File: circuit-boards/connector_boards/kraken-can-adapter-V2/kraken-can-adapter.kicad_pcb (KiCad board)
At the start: 2 copper layers, 44.3 x 25.3 mm, 4 parts, among them J1 CAN, J2 CAN, J3 CAN_L, J4 CAN_H

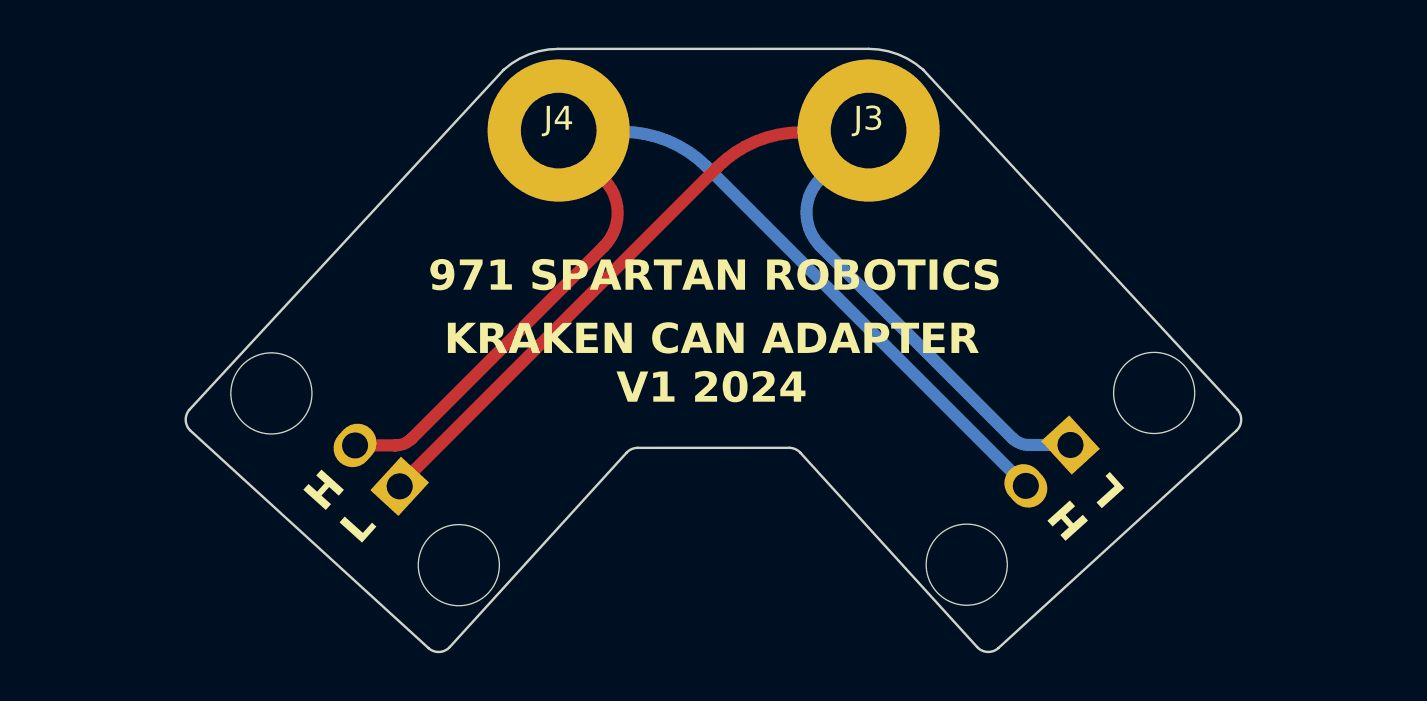
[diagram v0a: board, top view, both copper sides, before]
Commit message: Kraken Can V2
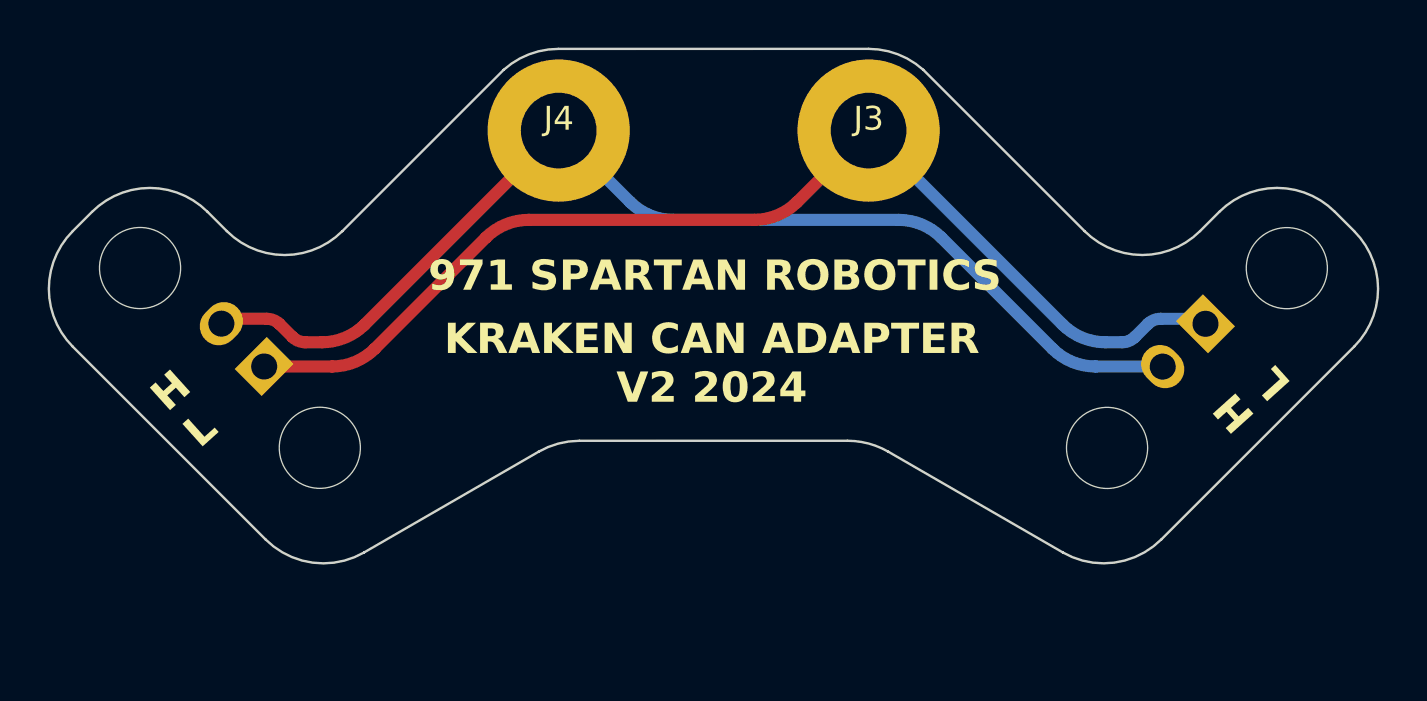
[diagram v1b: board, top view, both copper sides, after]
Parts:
- moved J2 34.5 mm to (126.9, 118.5), turned to -135 degrees
- moved J1 34.0 mm to (87.4, 120.3), turned to 135 degrees
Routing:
- net /CAN_L: track 45.3 -> 47.2 mm
- net /CAN_H: track 45.5 -> 47.2 mm
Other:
- board size 44.3 x 25.3 mm -> 55.8 x 21.6 mm
- board text added: "KRAKEN CAN ADAPTER V2 2024"
- board text removed: "KRAKEN CAN ADAPTER V1 2024"
